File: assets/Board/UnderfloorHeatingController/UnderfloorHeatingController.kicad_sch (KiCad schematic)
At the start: 10 parts, among them J2 Screw_Terminal_01x03, J3 Screw_Terminal_01x03, U2 Waveshare_ESP32-S3-Tiny

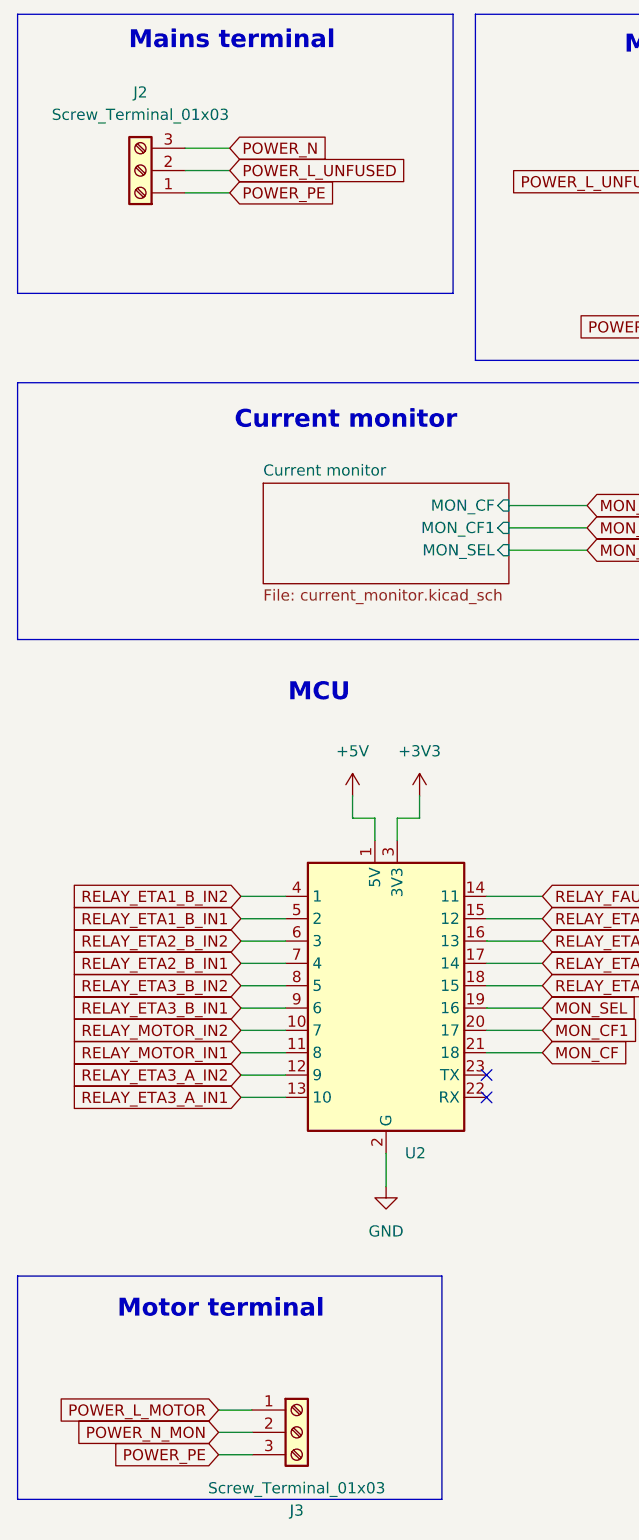
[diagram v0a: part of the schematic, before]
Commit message: Improved routing and layout.
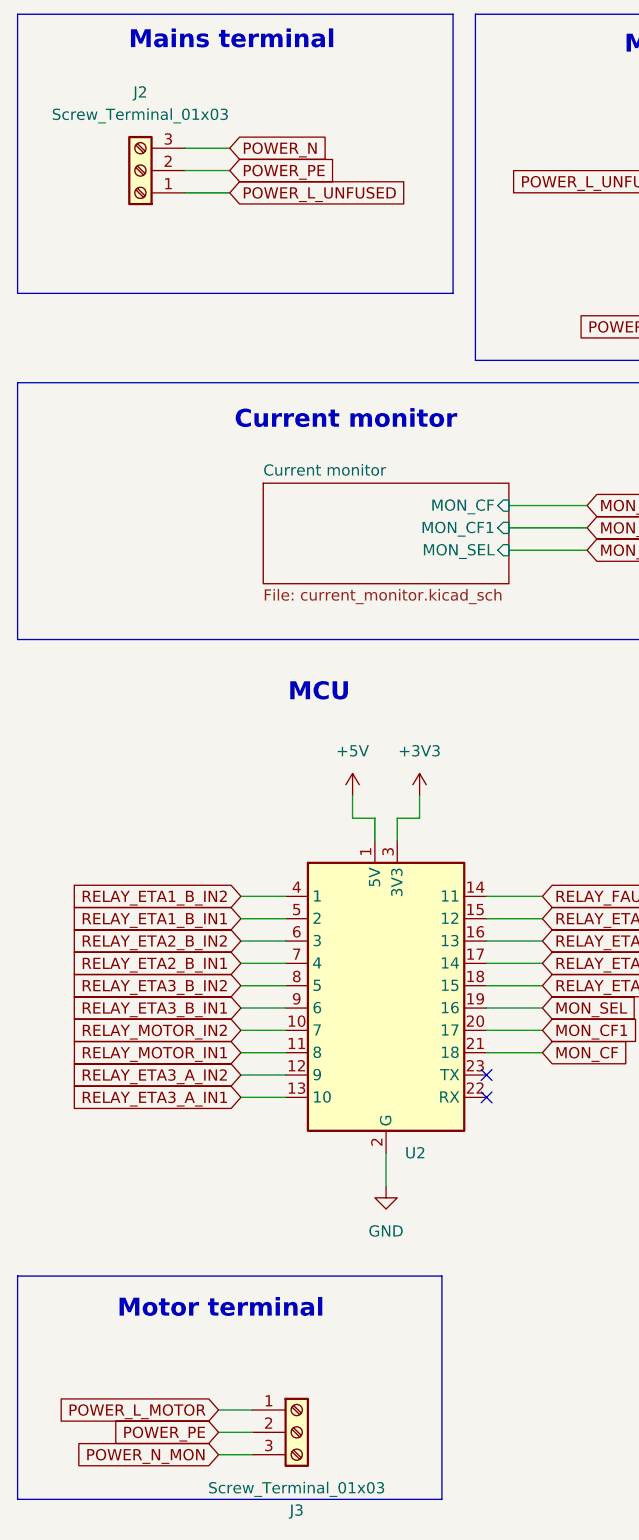
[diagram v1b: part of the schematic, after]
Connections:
- net POWER_L_UNFUSED: now also J2.1 (Pin_1); no longer J2.2 (Pin_2)
- net POWER_N_MON: now also J3.3 (Pin_3); no longer J3.2 (Pin_2)
- net POWER_PE: now also J2.2 (Pin_2), J3.2 (Pin_2); no longer J2.1 (Pin_1), J3.3 (Pin_3)
